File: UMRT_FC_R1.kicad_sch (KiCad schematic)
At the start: 1 part, among them J11 USB_A

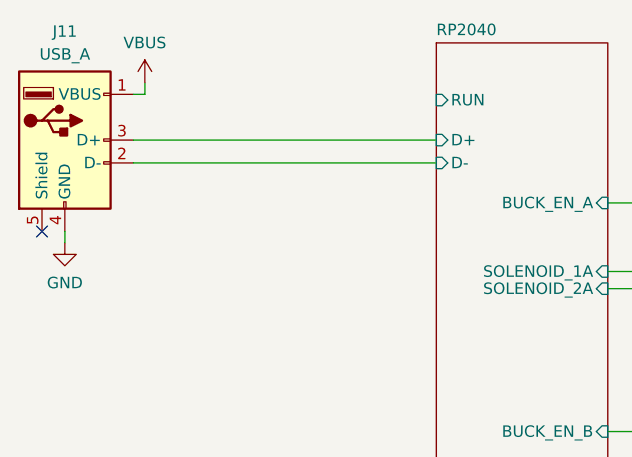
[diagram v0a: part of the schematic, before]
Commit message: added some notes and PDF
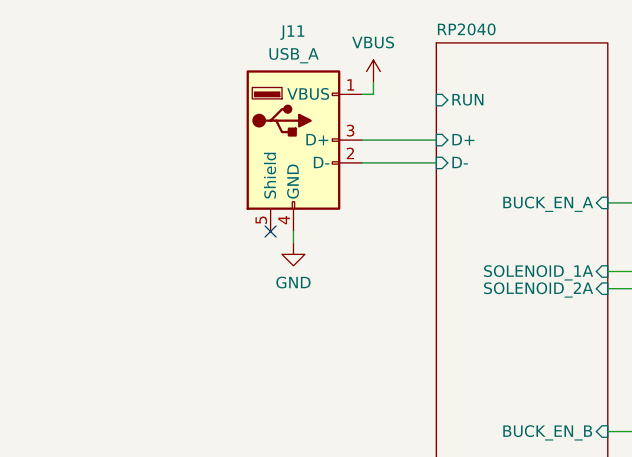
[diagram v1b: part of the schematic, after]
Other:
- moved on the sheet: J11
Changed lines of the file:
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@@
 (kicad_sch (version 20230121) (generator eeschema)
   (paper "A4")
-  (no_connect (at 70.485 78.105))
+  (no_connect (at 95.885 78.105))
   (wire (pts (xy 158.75 106.045) (xy 171.45 106.045))
     (stroke (width 0) (type default))
@@
     (stroke (width 0) (type default))
   )
-  (wire (pts (xy 80.645 67.945) (xy 114.3 67.945))
-    (stroke (width 0) (type default))
-  )
   (wire (pts (xy 133.35 100.33) (xy 139.7 100.33))
     (stroke (width 0) (type default))
@@
     (stroke (width 0) (type default))
   )
-  (wire (pts (xy 81.915 61.595) (xy 81.915 62.865))
+  (wire (pts (xy 107.315 61.595) (xy 107.315 62.865))
     (stroke (width 0) (type default))
   )
-  (wire (pts (xy 73.025 78.105) (xy 73.025 79.375))
+  (wire (pts (xy 98.425 78.105) (xy 98.425 79.375))
     (stroke (width 0) (type default))
   )
@@
     (stroke (width 0) (type default))
   )
+  (wire (pts (xy 106.045 70.485) (xy 114.3 70.485))
+    (stroke (width 0) (type default))
+  )
   (wire (pts (xy 133.35 136.525) (xy 171.45 136.525))
     (stroke (width 0) (type default))
@@
     (stroke (width 0) (type default))
   )
-  (wire (pts (xy 80.645 70.485) (xy 114.3 70.485))
-    (stroke (width 0) (type default))
-  )
-  (wire (pts (xy 80.645 62.865) (xy 81.915 62.865))
+  (wire (pts (xy 106.045 62.865) (xy 107.315 62.865))
     (stroke (width 0) (type default))
   )
@@
     (stroke (width 0) (type default))
   )
+  (wire (pts (xy 106.045 67.945) (xy 114.3 67.945))
+    (stroke (width 0) (type default))
+  )
   (wire (pts (xy 158.75 78.74) (xy 171.45 78.74))
     (stroke (width 0) (type default))
   )
-  (symbol (lib_id "power:GND") (at 73.025 79.375 0) (unit 1)
+  (symbol (lib_id "power:GND") (at 98.425 79.375 0) (unit 1)
     (in_bom yes) (on_board yes) (dnp no) (fields_autoplaced)
-    (property "Reference" "#PWR058" (at 73.025 85.725 0)
+    (property "Reference" "#PWR058" (at 98.425 85.725 0)
       (effects (font (size 1.27 1.27)) hide)
     )
-    (property "Value" "GND" (at 73.025 83.82 0)
+    (property "Value" "GND" (at 98.425 83.82 0)
       (effects (font (size 1.27 1.27)))
     )
-    (property "Footprint" "" (at 73.025 79.375 0)
+    (property "Footprint" "" (at 98.425 79.375 0)
       (effects (font (size 1.27 1.27)) hide)
     )
-    (property "Datasheet" "" (at 73.025 79.375 0)
+    (property "Datasheet" "" (at 98.425 79.375 0)
       (effects (font (size 1.27 1.27)) hide)
     )
@@
     )
   )
-  (symbol (lib_id "power:VBUS") (at 81.915 61.595 0) (unit 1)
+  (symbol (lib_id "power:VBUS") (at 107.315 61.595 0) (unit 1)
     (in_bom yes) (on_board yes) (dnp no) (fields_autoplaced)
-    (property "Reference" "#PWR049" (at 81.915 65.405 0)
+    (property "Reference" "#PWR049" (at 107.315 65.405 0)
       (effects (font (size 1.27 1.27)) hide)
     )
-    (property "Value" "VBUS" (at 81.915 57.15 0)
+    (property "Value" "VBUS" (at 107.315 57.15 0)
       (effects (font (size 1.27 1.27)))
     )
-    (property "Footprint" "" (at 81.915 61.595 0)
+    (property "Footprint" "" (at 107.315 61.595 0)
       (effects (font (size 1.27 1.27)) hide)
     )
-    (property "Datasheet" "" (at 81.915 61.595 0)
+    (property "Datasheet" "" (at 107.315 61.595 0)
       (effects (font (size 1.27 1.27)) hide)
     )
@@
     )
   )
-  (symbol (lib_id "Connector:USB_A") (at 73.025 67.945 0) (unit 1)
+  (symbol (lib_id "Connector:USB_A") (at 98.425 67.945 0) (unit 1)
     (in_bom yes) (on_board yes) (dnp no) (fields_autoplaced)
-    (property "Reference" "J11" (at 73.025 55.88 0)
+    (property "Reference" "J11" (at 98.425 55.88 0)
       (effects (font (size 1.27 1.27)))
     )
-    (property "Value" "USB_A" (at 73.025 58.42 0)
+    (property "Value" "USB_A" (at 98.425 58.42 0)
       (effects (font (size 1.27 1.27)))
     )
-    (property "Footprint" "" (at 76.835 69.215 0)
+    (property "Footprint" "" (at 102.235 69.215 0)
       (effects (font (size 1.27 1.27)) hide)
     )
-    (property "Datasheet" " ~" (at 76.835 69.215 0)
+    (property "Datasheet" " ~" (at 102.235 69.215 0)
       (effects (font (size 1.27 1.27)) hide)
     )
